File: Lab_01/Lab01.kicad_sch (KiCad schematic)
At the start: 0 parts

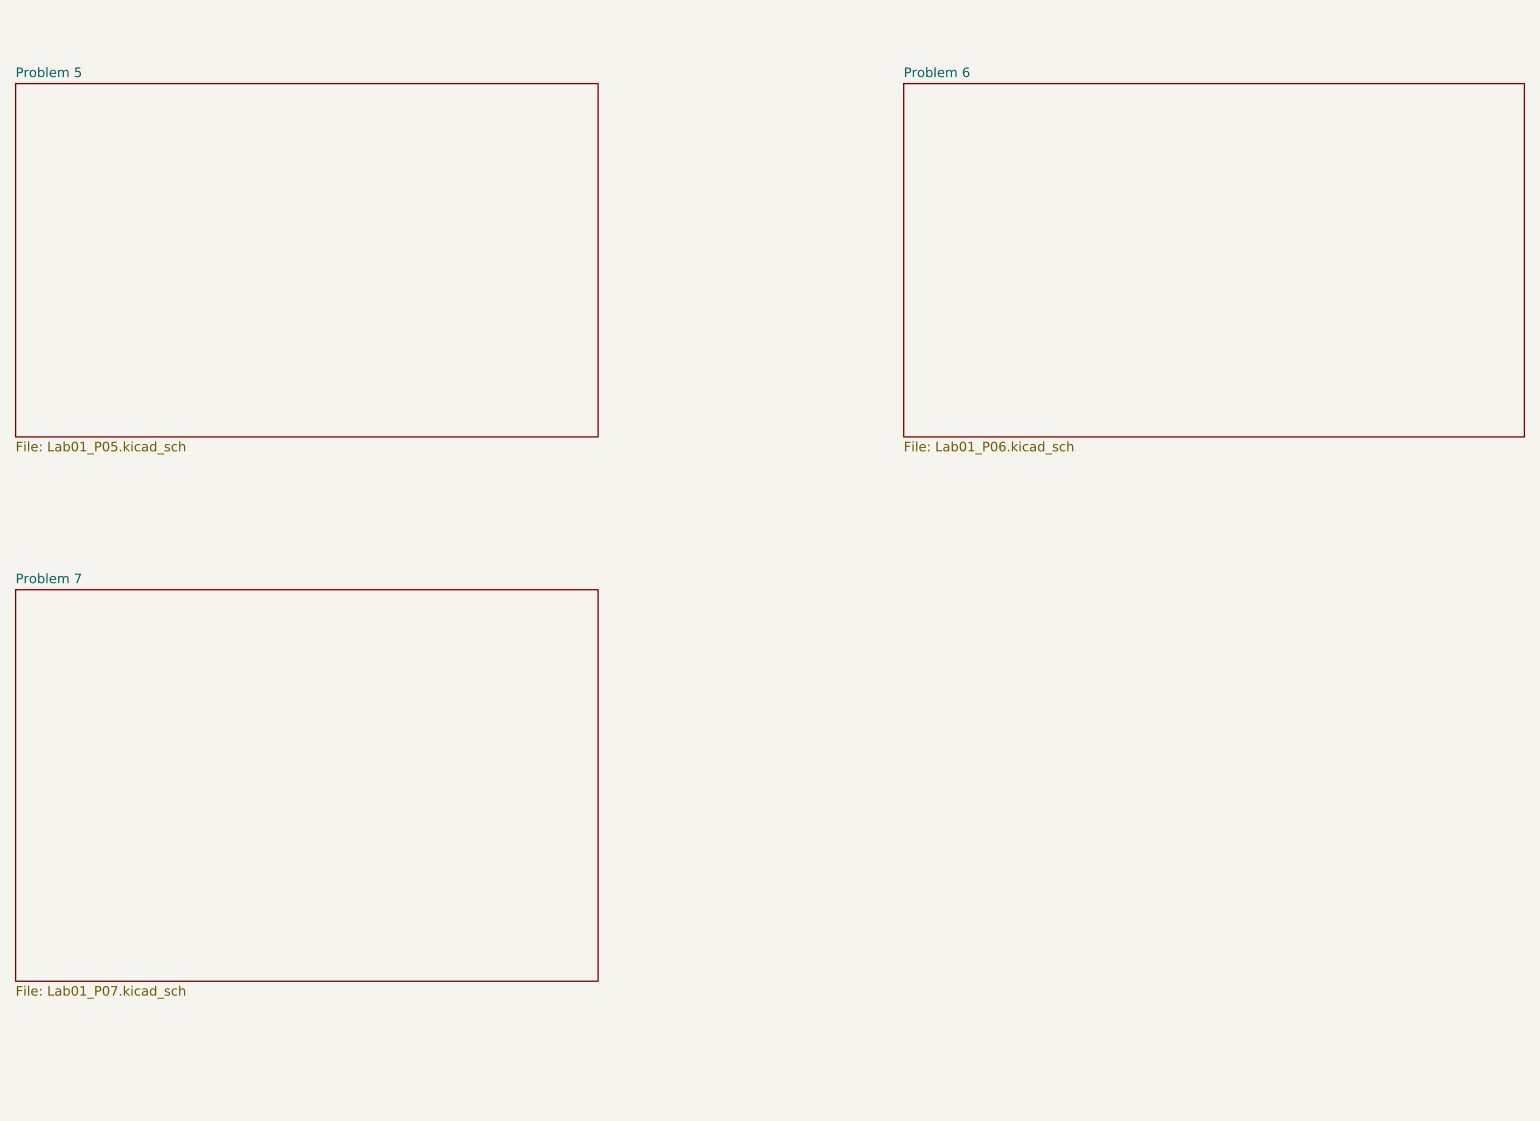
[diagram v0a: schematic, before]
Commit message: Edit up to Question 9
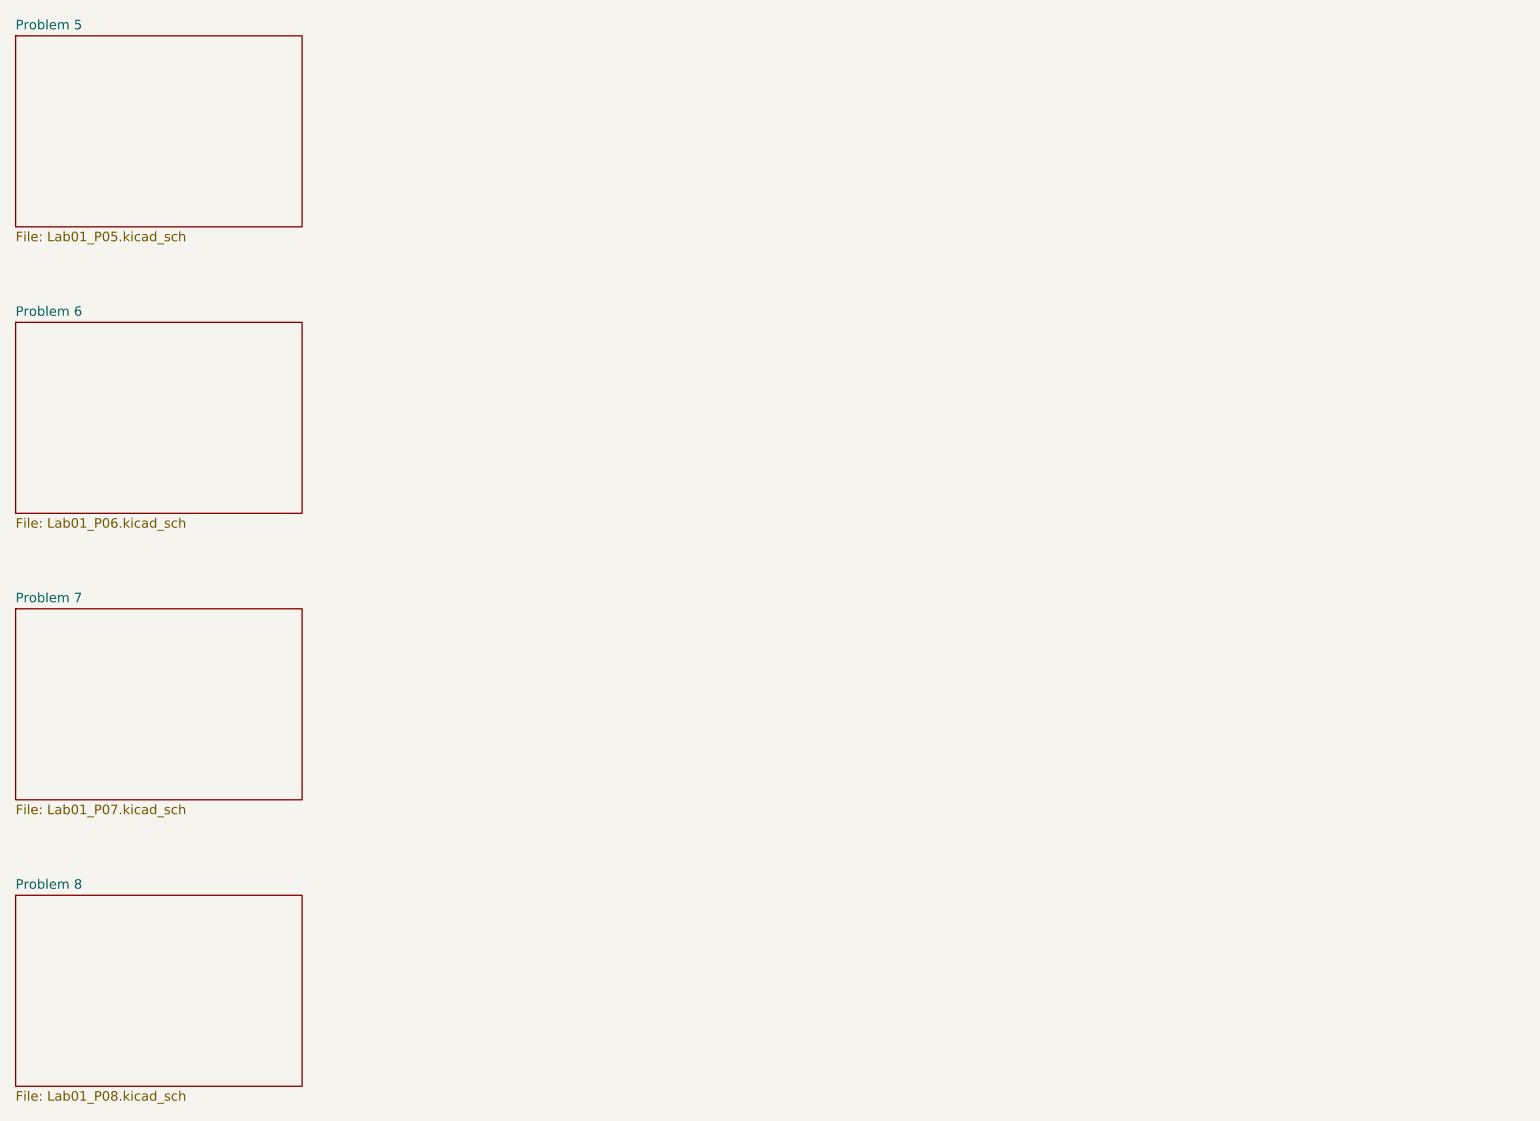
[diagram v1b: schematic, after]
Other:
- added sheet Problem 8 (Lab01_P08.kicad_sch)
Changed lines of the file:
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@@
     (company "Jim Horwitz & Mark Vaughn, Jork Incorporated")
   )
-  (sheet (at 38.1 99.06) (size 77.47 52.07) (fields_autoplaced)
+  (sheet (at 38.1 101.6) (size 38.1 25.4) (fields_autoplaced)
     (stroke (width 0.1524) (type solid))
     (fill (color 0 0 0 0.0000))
-    (property "Sheetname" "Problem 7" (at 38.1 98.3484 0)
+    (property "Sheetname" "Problem 7" (at 38.1 100.8884 0)
       (effects (font (size 1.27 1.27)) (justify left bottom))
     )
-    (property "Sheetfile" "Lab01_P07.kicad_sch" (at 38.1 151.7146 0)
+    (property "Sheetfile" "Lab01_P07.kicad_sch" (at 38.1 127.5846 0)
       (effects (font (size 1.27 1.27)) (justify left top))
     )
@@
     )
   )
-  (sheet (at 38.1 31.75) (size 77.47 46.99) (fields_autoplaced)
+  (sheet (at 38.1 139.7) (size 38.1 25.4) (fields_autoplaced)
     (stroke (width 0.1524) (type solid))
     (fill (color 0 0 0 0.0000))
-    (property "Sheetname" "Problem 5" (at 38.1 31.0384 0)
+    (property "Sheetname" "Problem 8" (at 38.1 138.9884 0)
       (effects (font (size 1.27 1.27)) (justify left bottom))
     )
-    (property "Sheetfile" "Lab01_P05.kicad_sch" (at 38.1 79.3246 0)
+    (property "Sheetfile" "Lab01_P08.kicad_sch" (at 38.1 165.6846 0)
+      (effects (font (size 1.27 1.27)) (justify left top))
+    )
+    (instances
+      (project "Lab01"
+        (path "/f5e37932-d66b-45bd-afc2-f24a1a74700d" (page "5"))
+      )
+    )
+  )
+  (sheet (at 38.1 25.4) (size 38.1 25.4) (fields_autoplaced)
+    (stroke (width 0.1524) (type solid))
+    (fill (color 0 0 0 0.0000))
+    (property "Sheetname" "Problem 5" (at 38.1 24.6884 0)
+      (effects (font (size 1.27 1.27)) (justify left bottom))
+    )
+    (property "Sheetfile" "Lab01_P05.kicad_sch" (at 38.1 51.3846 0)
       (effects (font (size 1.27 1.27)) (justify left top))
     )
@@
     )
   )
-  (sheet (at 156.21 31.75) (size 82.55 46.99) (fields_autoplaced)
+  (sheet (at 38.1 63.5) (size 38.1 25.4) (fields_autoplaced)
     (stroke (width 0.1524) (type solid))
     (fill (color 0 0 0 0.0000))
-    (property "Sheetname" "Problem 6" (at 156.21 31.0384 0)
+    (property "Sheetname" "Problem 6" (at 38.1 62.7884 0)
       (effects (font (size 1.27 1.27)) (justify left bottom))
     )
-    (property "Sheetfile" "Lab01_P06.kicad_sch" (at 156.21 79.3246 0)
+    (property "Sheetfile" "Lab01_P06.kicad_sch" (at 38.1 89.4846 0)
       (effects (font (size 1.27 1.27)) (justify left top))
     )
